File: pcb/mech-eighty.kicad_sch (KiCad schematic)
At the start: 22 parts, among them J1 JSTx04, SW1 Boot0, SW2 Reset, U1 STM32F103C8T6, U2 AMS1117-3.3, Y1 8MHz

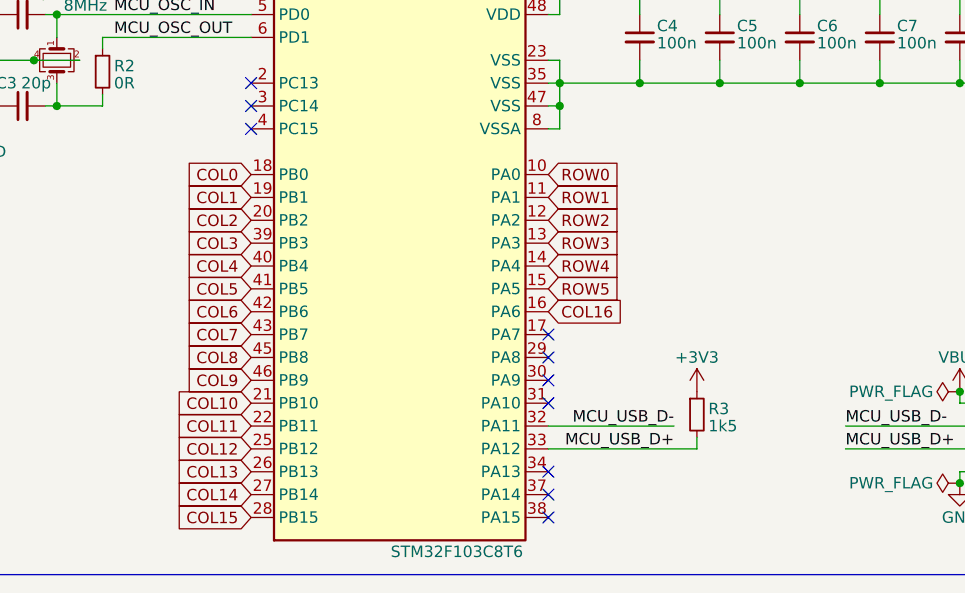
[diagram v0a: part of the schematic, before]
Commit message: Routing completed
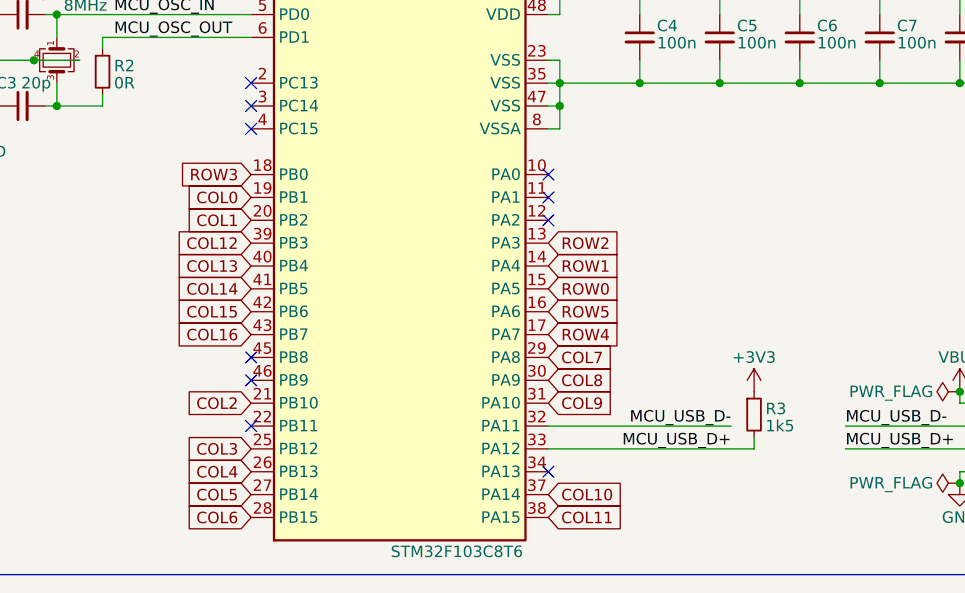
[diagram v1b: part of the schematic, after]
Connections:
- net COL0: now also U1.19 (PB1); no longer U1.18 (PB0)
- net COL1: now also U1.20 (PB2); no longer U1.19 (PB1)
- net COL10: now also U1.37 (PA14); no longer U1.21 (PB10)
- net COL11: now also U1.38 (PA15); no longer U1.22 (PB11)
- net COL12: now also U1.39 (PB3); no longer U1.25 (PB12)
- net COL13: now also U1.40 (PB4); no longer U1.26 (PB13)
- net COL14: now also U1.41 (PB5); no longer U1.27 (PB14)
- net COL15: now also U1.42 (PB6); no longer U1.28 (PB15)
- net COL16: now also U1.43 (PB7); no longer U1.16 (PA6)
- net COL2: now also U1.21 (PB10); no longer U1.20 (PB2)
- net COL3: now also U1.25 (PB12); no longer U1.39 (PB3)
- net COL4: now also U1.26 (PB13); no longer U1.40 (PB4)
- net COL5: now also U1.27 (PB14); no longer U1.41 (PB5)
- net COL6: now also U1.28 (PB15); no longer U1.42 (PB6)
- net COL7: now also U1.29 (PA8); no longer U1.43 (PB7)
- net COL8: now also U1.30 (PA9); no longer U1.45 (PB8)
- net COL9: now also U1.31 (PA10); no longer U1.46 (PB9)
- net ROW0: now also U1.15 (PA5); no longer U1.10 (PA0)
- net ROW1: now also U1.14 (PA4); no longer U1.11 (PA1)
- net ROW2: now also U1.13 (PA3); no longer U1.12 (PA2)
- net ROW3: now also U1.18 (PB0); no longer U1.13 (PA3)
- net ROW4: now also U1.17 (PA7); no longer U1.14 (PA4)
- net ROW5: now also U1.16 (PA6); no longer U1.15 (PA5)
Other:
- moved on the sheet: R3

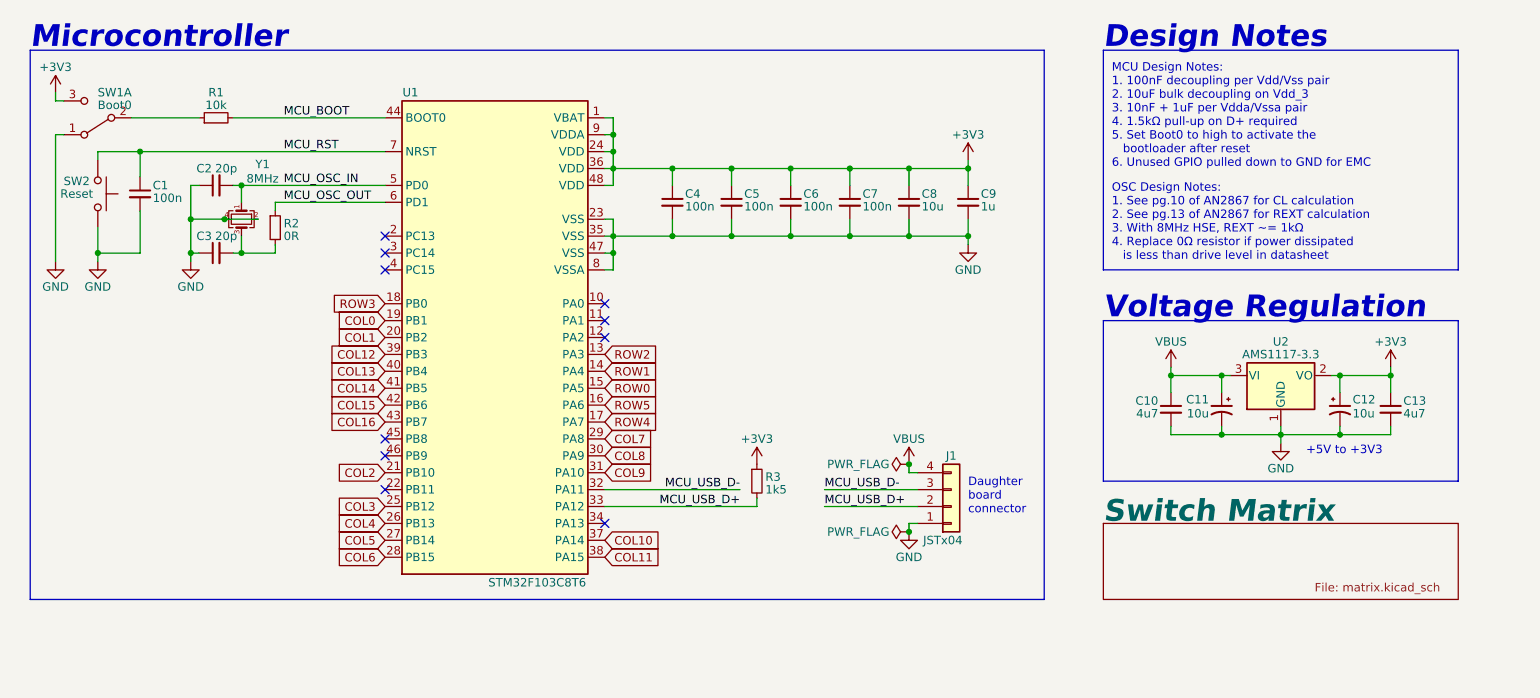
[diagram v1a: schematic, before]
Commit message: update
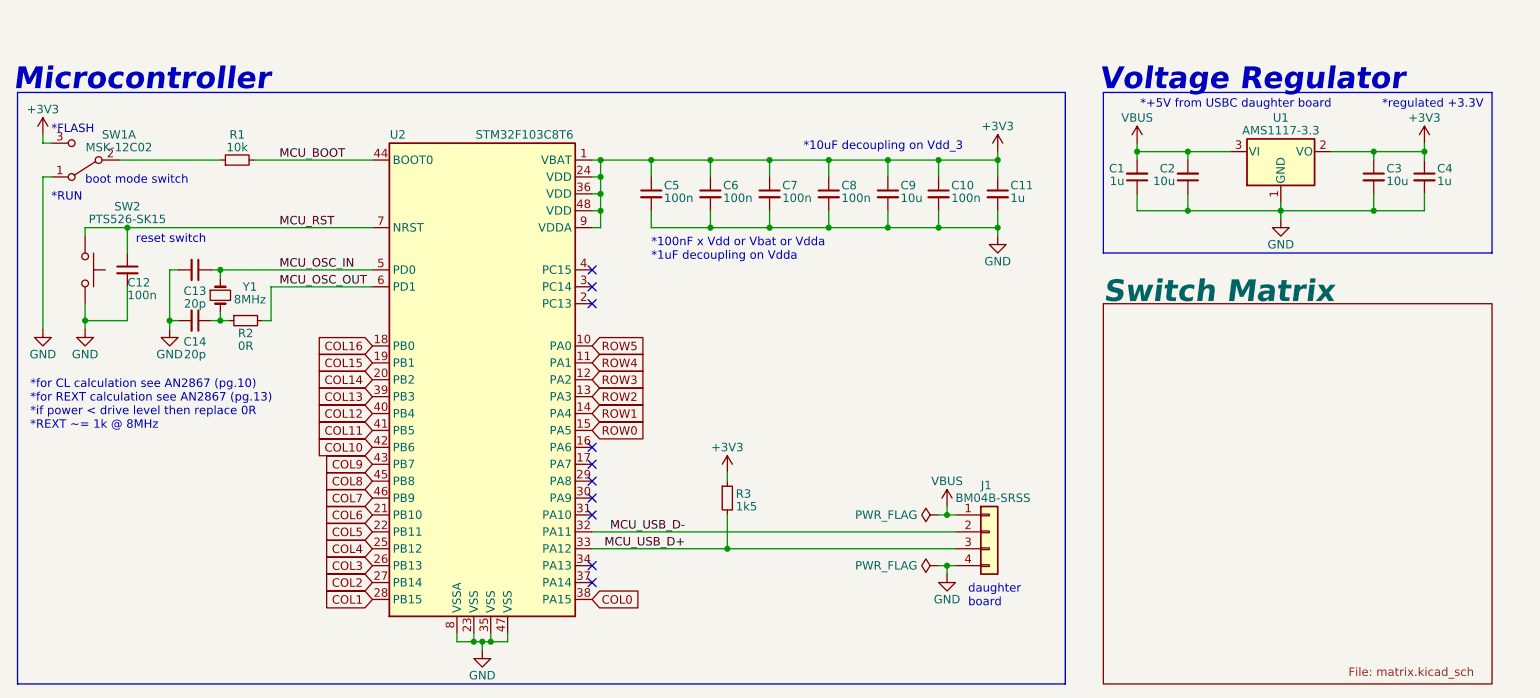
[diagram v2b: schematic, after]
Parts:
- removed C11, C12: 10u, capacitors:C-3216-18A, symbol Device:C_Polarized_Small_US
- removed J1: JSTx04, connectors:JST-SM04B-GHS-TB_1x4P, symbol Connector-Generic:Conn_01x04
- removed SW1: Boot0, switches:SW-SPDT-PCM12, symbol Switches:SW_DPDT_x2
- removed SW2: Reset, switches:SW-SPST-B3U-1000P, symbol Switches:SW_Push
- removed U1: STM32F103C8T6, packages:LQFP-48, symbol MCU-ST-STM32F103:STM32F103C8T6
- removed U2: AMS1117-3.3, packages:SOT-223, symbol Regulator-Linear:AMS1117-3.3
- removed Y1: 8MHz, crystals:Crystal-SMD-3225-4P, symbol Device:Crystal_GND24_Small
- added C11: 1u, Capacitor_SMD:C_0805_2012Metric, symbol Device:C_Small
- added C12: 100n, Capacitor_SMD:C_0603_1608Metric, symbol Device:C_Small
- added C14: 20p, Capacitor_SMD:C_0603_1608Metric, symbol Device:C_Small
- added J1: BM04B-SRSS, Connector_JST:JST_SH_SM04B-SRSS-TB_1x04-1MP_P1.00mm_Horizontal, symbol Connector_Generic:Conn_01x04
- added SW1: MSK-12C02, Button_Switch_SMD:SW_SPDT_PCM12, symbol Button_Switch:SW_DPDT_x2
- added SW2: PTS526-SK15, Button_Switch_SMD:SW_PTS526_SM08_SMTR2_LFS, symbol Button_Switch:SW_Push
- added U1: AMS1117-3.3, Package_TO_SOT_SMD:SOT-223-3_TabPin2, symbol Regulator_Linear:AMS1117-3.3
- added U2: STM32F103C8T6, Package_QFP:LQFP-48_7x7mm_P0.5mm, symbol Custom_Components:STM32F103C8T6
- added Y1: 8MHz, Crystal:Crystal_SMD_HC49-SD, symbol Device:Crystal_Small
- C1, C4: value 100n -> 1u; footprint capacitors:C-0603-1608 -> Capacitor_SMD:C_0805_2012Metric
- C10: value 4u7 -> 100n; footprint capacitors:C-0805-2012 -> Capacitor_SMD:C_0603_1608Metric
- C13: value 4u7 -> 20p; footprint capacitors:C-0805-2012 -> Capacitor_SMD:C_0603_1608Metric
- C2, C3: value 20p -> 10u; footprint capacitors:C-0603-1608 -> Capacitor_SMD:C_0805_2012Metric
- C5, C6, C7: footprint capacitors:C-0603-1608 -> Capacitor_SMD:C_0603_1608Metric
- C8: value 10u -> 100n; footprint capacitors:C-0805-2012 -> Capacitor_SMD:C_0603_1608Metric
- C9: value 1u -> 10u; footprint capacitors:C-0805-2012 -> Capacitor_SMD:C_0805_2012Metric
- R1, R2, R3: footprint resistors:R-0603-1608 -> Resistor_SMD:R_0603_1608Metric
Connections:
- net +3V3: now also C10.1, C3.1, C11.1, SW1.3 (C), U1.2 (VO), U2.1 (VBAT), U2.24 (VDD), U2.36 (VDD), U2.48 (VDD), U2.9 (VDDA); no longer C13.1
- net COL0: now also U2.38 (PA15)
- net COL1: now also U2.28 (PB15)
- net COL10: now also U2.42 (PB6)
- net COL11: now also U2.41 (PB5)
- net COL12: now also U2.40 (PB4)
- net COL13: now also U2.39 (PB3)
- net COL14: now also U2.20 (PB2)
- net COL15: now also U2.19 (PB1)
- net COL16: now also U2.18 (PB0)
- net COL2: now also U2.27 (PB14)
- net COL3: now also U2.26 (PB13)
- net COL4: now also U2.25 (PB12)
- net COL5: now also U2.22 (PB11)
- net COL6: now also U2.21 (PB10)
- net COL7: now also U2.46 (PB9)
- net COL8: now also U2.45 (PB8)
- net COL9: now also U2.43 (PB7)
- net GND: now also C1.1, C3.2, C11.2, C12.2, C14.2, J1.4 (Pin_4), SW1.1 (A), SW2.2, U1.1 (GND), U2.23 (VSS), U2.35 (VSS), U2.47 (VSS), U2.8 (VSSA); no longer C1.2, C3.1
- net MCU_BOOT: now also U2.44 (BOOT0)
- net MCU_OSC_IN: now also C13.1, U2.5 (PD0), Y1.1; no longer C2.2
- net MCU_OSC_OUT: now also R2.2, U2.6 (PD1); no longer R2.1
- net MCU_RST: now also C12.1, SW2.1, U2.7 (NRST); no longer C1.1
- net MCU_USB_D+: now also J1.3 (Pin_3), U2.33 (PA12)
- net MCU_USB_D-: now also J1.2 (Pin_2), U2.32 (PA11)
- net ROW0: now also U2.15 (PA5)
- net ROW1: now also U2.14 (PA4)
- net ROW2: now also U2.13 (PA3)
- net ROW3: now also U2.12 (PA2)
- net ROW4: now also U2.11 (PA1)
- net ROW5: now also U2.10 (PA0)
- net VBUS: now also C1.2, C2.2, J1.1 (Pin_1), U1.3 (VI); no longer C10.1
- net at R1.1: now also SW1.2 (B)
- new net: C14.1, R2.1, Y1.2
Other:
- note added: "*+5V from USBC daughter board"
- note added: "*100nF x Vdd or Vbat or Vdda *1uF decoupling on Vdda"
- note added: "*10uF decoupling on Vdd_3"
- note added: "*FLASH"
- note added: "*RUN"
- note added: "*for CL calculation see AN2867 (pg.10) *for REXT calculation see AN2867 (pg.13) *if power < drive level then replace 0R *REXT ~= 1k @ 8MHz"
- note added: "*regulated +3.3V"
- note added: "Voltage Regulator"
- note added: "boot mode switch"
- note added: "daughter board"
- note added: "reset switch"
- note removed: "+5V to +3V3"
- note removed: "Daughter board connector"
- note removed: "Design Notes"
- note removed: "MCU Design Notes: 1. 100nF decoupling per Vdd/Vss pair 2. 10uF bulk decoupling on Vdd_3 3. 10nF + 1uF per Vdda/Vssa pair 4. 1.5kΩ pull-up on D+ required 5. Set Boot0 to high to activate the bootloader after reset 6. Unused GPIO pulled down to GND for EMC"
- note removed: "OSC Design Notes: 1. See pg.10 of AN2867 for CL calculation 2. See pg.13 of AN2867 for REXT calculation 3. With 8MHz HSE, REXT ~= 1kΩ 4. Replace 0Ω resistor if power dissipated is less than drive level in datasheet"
- note removed: "Voltage Regulation"
- title: mech-eighty -> Mech Eighty
